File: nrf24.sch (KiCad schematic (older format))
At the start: 1 part, among them U11 NRF24L01_Breakout

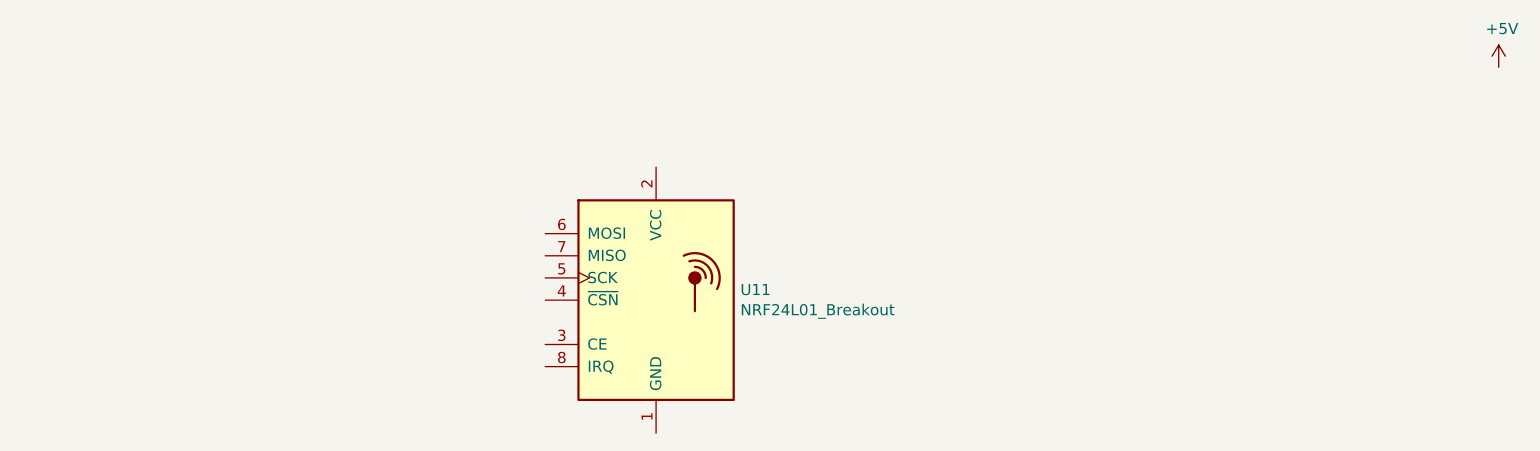
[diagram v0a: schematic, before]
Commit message: finish board
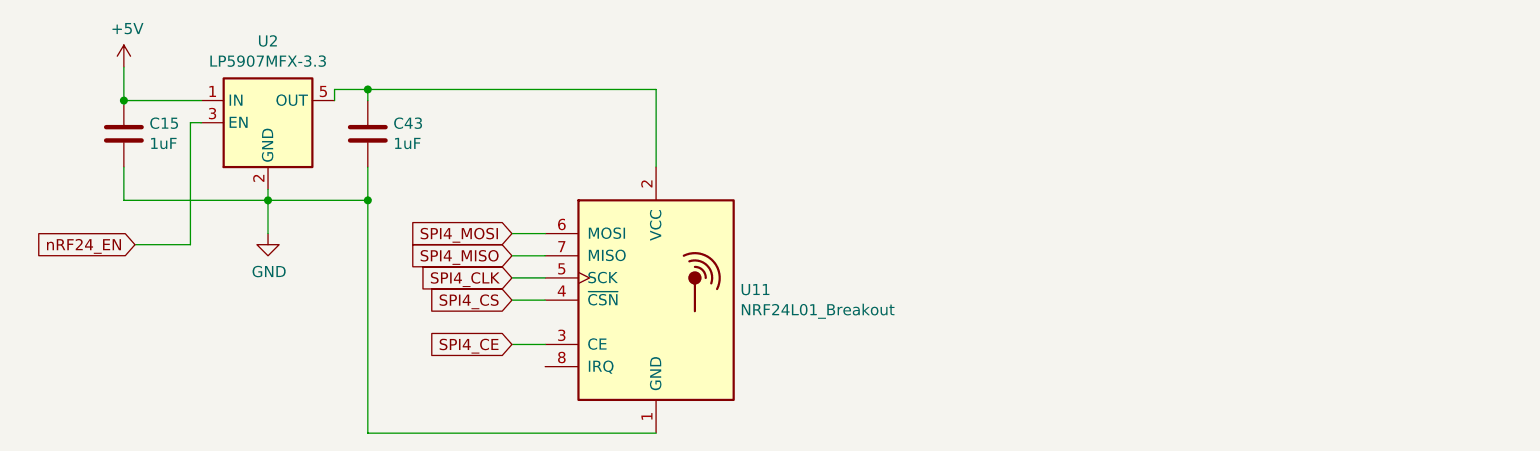
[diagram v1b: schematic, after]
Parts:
- added C15, C43: 1uF, Capacitor_SMD:C_0603_1608Metric_Pad1.05x0.95mm_HandSolder, symbol Device:C
- added U2: LP5907MFX-3.3, Package_TO_SOT_SMD:SOT-23-5, symbol Regulator_Linear:LP5907MFX-3.3
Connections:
- net +5V: now also C15.1, U2.1 (IN)
- net GND: now reaches U11.1 (GND)
- net GND: now also C15.2, C43.2, U2.2 (GND)
- net at U11.2 (VCC): now also C43.1, U2.5 (OUT)
- net SPI4_CE: now reaches U11.3 (CE)
- net SPI4_CS: now reaches U11.4 (~CSN)
- net SPI4_CLK: now reaches U11.5 (SCK)
- net SPI4_MOSI: now reaches U11.6 (MOSI)
- net SPI4_MISO: now reaches U11.7 (MISO)
- new net nRF24_EN: U2.3 (EN)
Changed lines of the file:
@@
+	1    0    0    -1
+$EndComp
+Text GLabel 3400 3500 0    50   Input ~ 0
+SPI4_MISO
+Text GLabel 3400 3400 0    50   Input ~ 0
+SPI4_MOSI
+Text GLabel 3400 3600 0    50   Input ~ 0
+SPI4_CLK
+Wire Wire Line
+	3550 3600 3400 3600
+Wire Wire Line
+	3550 3500 3400 3500
+Wire Wire Line
+	3550 3400 3400 3400
+Text GLabel 3400 3900 0    50   Input ~ 0
+SPI4_CE
+Text GLabel 3400 3700 0    50   Input ~ 0
+SPI4_CS
+Wire Wire Line
+	3400 3900 3550 3900
+Wire Wire Line
+	3550 3700 3400 3700
+$Comp
+L Device:C C?
+U 1 1 5F5DC7F7
+P 1650 2950
+AR Path="/5F5DC7F7" Ref="C?"  Part="1"
+AR Path="/5F569749/5F5DC7F7" Ref="C?"  Part="1"
+AR Path="/5F3218EE/5F5DC7F7" Ref="C?"  Part="1"
+AR Path="/5F584BC5/5F5DC7F7" Ref="C?"  Part="1"
+AR Path="/5F5AF088/5F5DC7F7" Ref="C?"  Part="1"
+AR Path="/5FD47887/5F5DC7F7" Ref="C15"  Part="1"
+F 0 "C15" H 1765 2996 50  0000 L CNN
+F 1 "1uF" H 1765 2905 50  0000 L CNN
+F 2 "Capacitor_SMD:C_0603_1608Metric_Pad1.05x0.95mm_HandSolder" H 1688 2800 50  0001 C CNN
+F 3 "~" H 1650 2950 50  0001 C CNN
+	1    1650 2950
+	1    0    0    -1
+$EndComp
+Wire Wire Line
+	2300 3250 2300 3400
+$Comp
+L power:GND #PWR?
+U 1 1 5F5DC7FE
+P 2300 3400
+AR Path="/5F3218EE/5F5DC7FE" Ref="#PWR?"  Part="1"
+AR Path="/5F5DC7FE" Ref="#PWR?"  Part="1"
+AR Path="/5F584BC5/5F5DC7FE" Ref="#PWR?"  Part="1"
+AR Path="/5F5AF088/5F5DC7FE" Ref="#PWR?"  Part="1"
+AR Path="/5FD47887/5F5DC7FE" Ref="#PWR0161"  Part="1"
+F 0 "#PWR0161" H 2300 3150 50  0001 C CNN
+F 1 "GND" H 2305 3227 50  0000 C CNN
+F 2 "" H 2300 3400 50  0001 C CNN
+F 3 "" H 2300 3400 50  0001 C CNN
+	1    2300 3400
 	1    0    0    -1
 $EndComp
 $Comp
-L power:+5V #PWR0161
-U 1 1 5FD4C9DA
-P 7850 2650
-F 0 "#PWR0161" H 7850 2500 50  0001 C CNN
-F 1 "+5V" H 7865 2823 50  0000 C CNN
-F 2 "" H 7850 2650 50  0001 C CNN
-F 3 "" H 7850 2650 50  0001 C CNN
-	1    7850 2650
+L power:+5V #PWR?
+U 1 1 5F5DC804
+P 1650 2650
+AR Path="/5F3218EE/5F5DC804" Ref="#PWR?"  Part="1"
+AR Path="/5F5DC804" Ref="#PWR?"  Part="1"
+AR Path="/5F584BC5/5F5DC804" Ref="#PWR?"  Part="1"
+AR Path="/5F5AF088/5F5DC804" Ref="#PWR?"  Part="1"
+AR Path="/5FD47887/5F5DC804" Ref="#PWR0183"  Part="1"
+F 0 "#PWR0183" H 1650 2500 50  0001 C CNN
+F 1 "+5V" H 1665 2823 50  0000 C CNN
+F 2 "" H 1650 2650 50  0001 C CNN
+F 3 "" H 1650 2650 50  0001 C CNN
+	1    1650 2650
 	1    0    0    -1
 $EndComp
+Wire Wire Line
+	1650 2800 1650 2650
+Connection ~ 1650 2800
+$Comp
+L Regulator_Linear:LP5907MFX-3.3 U?
+U 1 1 5F5DC80C
+P 2300 2900
+AR Path="/5F584BC5/5F5DC80C" Ref="U?"  Part="1"
+AR Path="/5FD47887/5F5DC80C" Ref="U2"  Part="1"
+F 0 "U2" H 2300 3267 50  0000 C CNN
+F 1 "LP5907MFX-3.3" H 2300 3176 50  0000 C CNN
+F 2 "Package_TO_SOT_SMD:SOT-23-5" H 2300 3250 50  0001 C CNN
+F 3 "http://www.ti.com/lit/ds/symlink/lp5907.pdf" H 2300 3400 50  0001 C CNN
+	1    2300 2900
+	1    0    0    -1
+$EndComp
+Connection ~ 2300 3250
+Wire Wire Line
+	1650 3250 2300 3250
+Wire Wire Line
+	2300 3250 2750 3250
+Wire Wire Line
+	2300 3250 2300 3200
+Wire Wire Line
+	1650 3100 1650 3250
+Wire Wire Line
+	1650 2800 2000 2800
+Wire Wire Line
+	1950 3450 1950 2900
+Wire Wire Line
+	1950 2900 2000 2900
+Wire Wire Line
+	4050 3100 4050 2750
+Wire Wire Line
+	4050 2750 2750 2750
+Wire Wire Line
+	2600 2750 2600 2800
+Wire Wire Line
+	2750 3250 2750 4300
+Wire Wire Line
+	2750 4300 4050 4300
+$Comp
+L Device:C C?
+U 1 1 5F5DE676
+P 2750 2950
+AR Path="/5F5DE676" Ref="C?"  Part="1"
+AR Path="/5F569749/5F5DE676" Ref="C?"  Part="1"
+AR Path="/5F3218EE/5F5DE676" Ref="C?"  Part="1"
+AR Path="/5F584BC5/5F5DE676" Ref="C?"  Part="1"
+AR Path="/5F5AF088/5F5DE676" Ref="C?"  Part="1"
+AR Path="/5FD47887/5F5DE676" Ref="C43"  Part="1"
+F 0 "C43" H 2865 2996 50  0000 L CNN
+F 1 "1uF" H 2865 2905 50  0000 L CNN
+F 2 "Capacitor_SMD:C_0603_1608Metric_Pad1.05x0.95mm_HandSolder" H 2788 2800 50  0001 C CNN
+F 3 "~" H 2750 2950 50  0001 C CNN
+	1    2750 2950
+	1    0    0    -1
+$EndComp
+Wire Wire Line
+	2750 3100 2750 3250
+Connection ~ 2750 3250
+Wire Wire Line
+	2750 2800 2750 2750
+Connection ~ 2750 2750
+Wire Wire Line
+	2750 2750 2600 2750
+Text GLabel 1700 3450 0    50   Input ~ 0
+nRF24_EN
+Wire Wire Line
+	1700 3450 1950 3450
 $EndSCHEMATC
